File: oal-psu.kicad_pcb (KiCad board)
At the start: 2 copper layers, 57 parts, among them J1 MAINS_LINE, J2 MAINS_NEUTRAL, J3 OUTPUT, P101 ENABLE_A, P2 OUTPUT_SELECT, P201 ENABLE_B, SW1 DPDT_SLIDE, SW102 VOLTAGE_A, SW202 VOLTAGE_B, T1 TALEMA 15/25VA, U101 TPS7A4700, U201 TPS7A4700

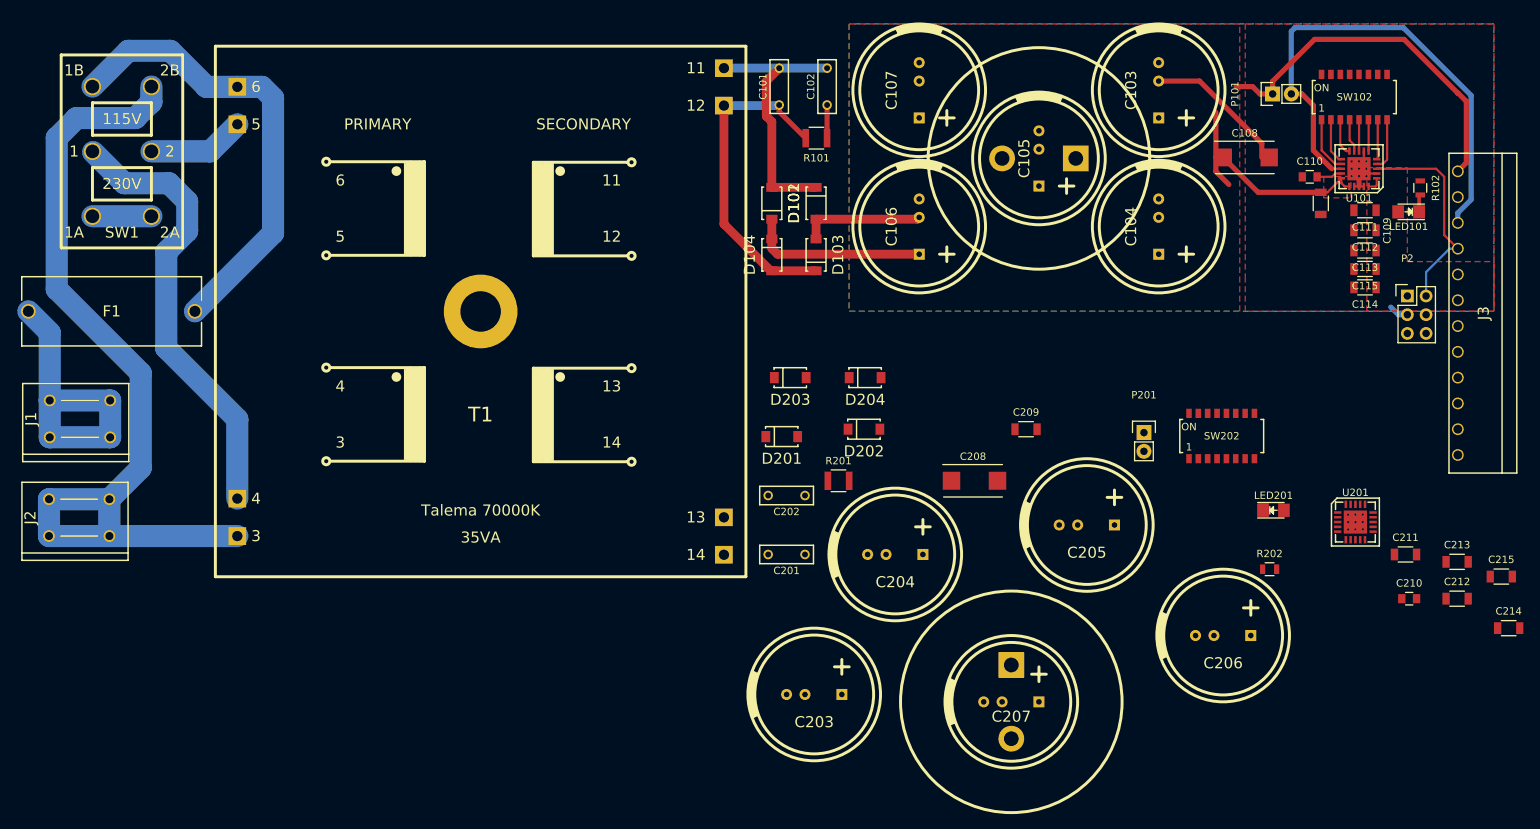
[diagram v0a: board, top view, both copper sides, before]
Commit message: board outline
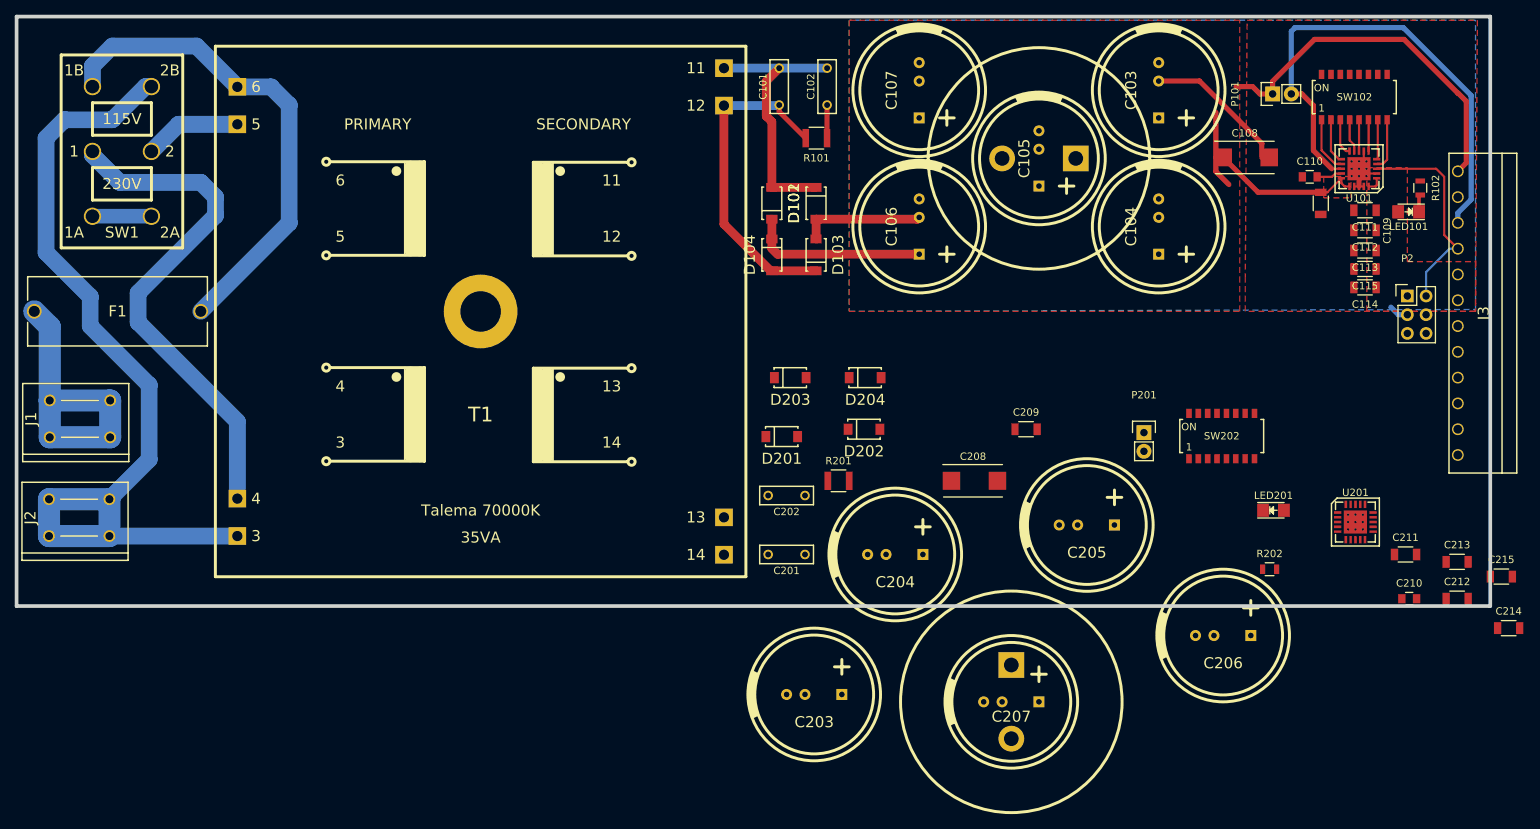
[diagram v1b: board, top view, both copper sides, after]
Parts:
- moved F1 0.80 mm to (45.7, 110.0)
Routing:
- net Net-(SW1-Pad5): track 61.1 -> 70.4 mm
- net Net-(F1-Pad2): track 62.5 -> 66.9 mm
- net NEUTRAL: track 116.3 -> 118.0 mm
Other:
- board outline added: 200 x 80 mm
- net class MAINS: trace_width 3 -> 2.28
